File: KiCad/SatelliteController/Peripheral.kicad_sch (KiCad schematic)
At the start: 8 parts, among them J15 CONN_AUDIO, J16 CONN_SPEAKER, J2 CONN_RS485, U2 24LC256, U6 DFPlayer, U7 LTC485CN8#PBF

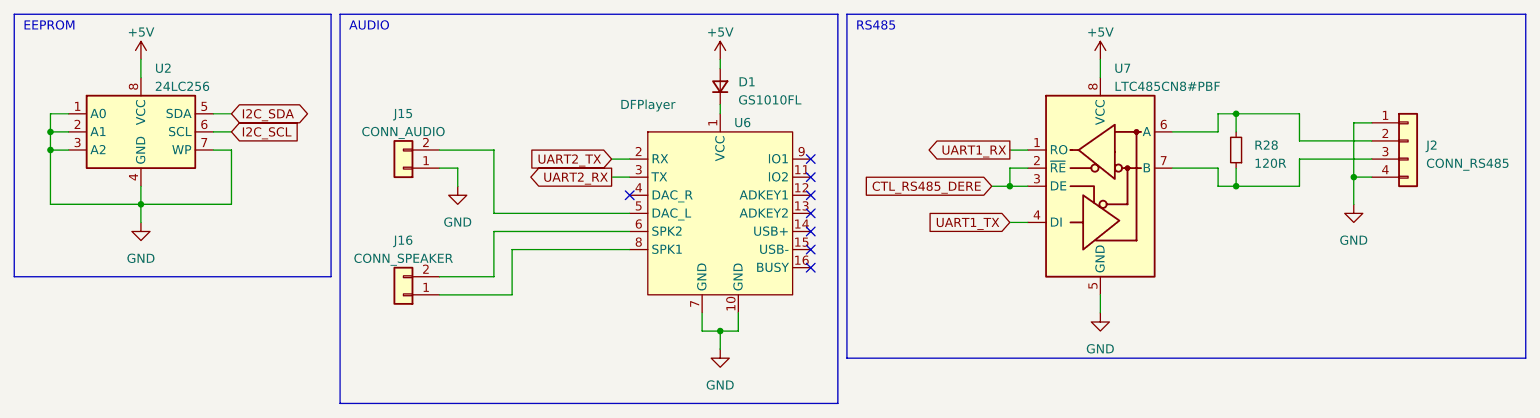
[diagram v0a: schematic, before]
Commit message: 音声完成を削除
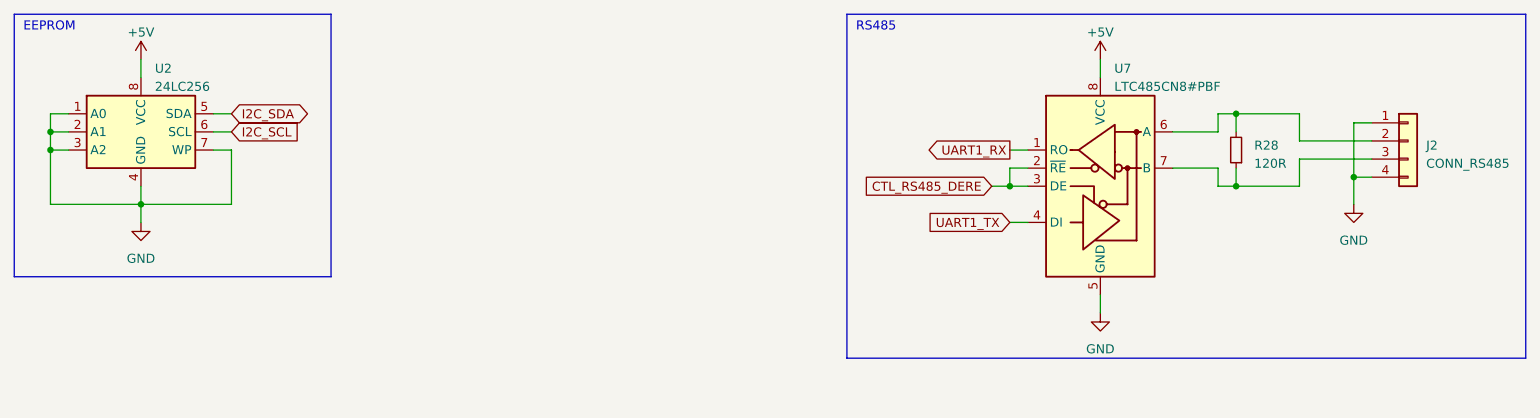
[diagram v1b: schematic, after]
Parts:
- removed D1: GS1010FL, Diode_SMD:D_SOD-123F, symbol Device:D_Small
- removed J15: CONN_AUDIO, TSRP_TerminalBlock_Alphaplus:TB401-1-2-E, symbol Connector_Generic:Conn_01x02
- removed J16: CONN_SPEAKER, TSRP_TerminalBlock_Alphaplus:TB401-1-2-E, symbol Connector_Generic:Conn_01x02
- removed U6: DFPlayer, TSRP_Module:DFPlayer-mini, symbol TSRP_Module:DFPlayer-mini
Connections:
- no-connect marks 8 -> 0
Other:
- note removed: "AUDIO"
